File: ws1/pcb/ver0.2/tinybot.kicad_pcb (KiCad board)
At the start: 2 copper layers, 46.7 x 46.2 mm, 19 parts, among them IC1 ATTINY84-P, P1 PWR, P2 Pins Breakout, P3 ICSP, P4 M1, P5 M2, U1 LD1117S33TR, U2 L293D

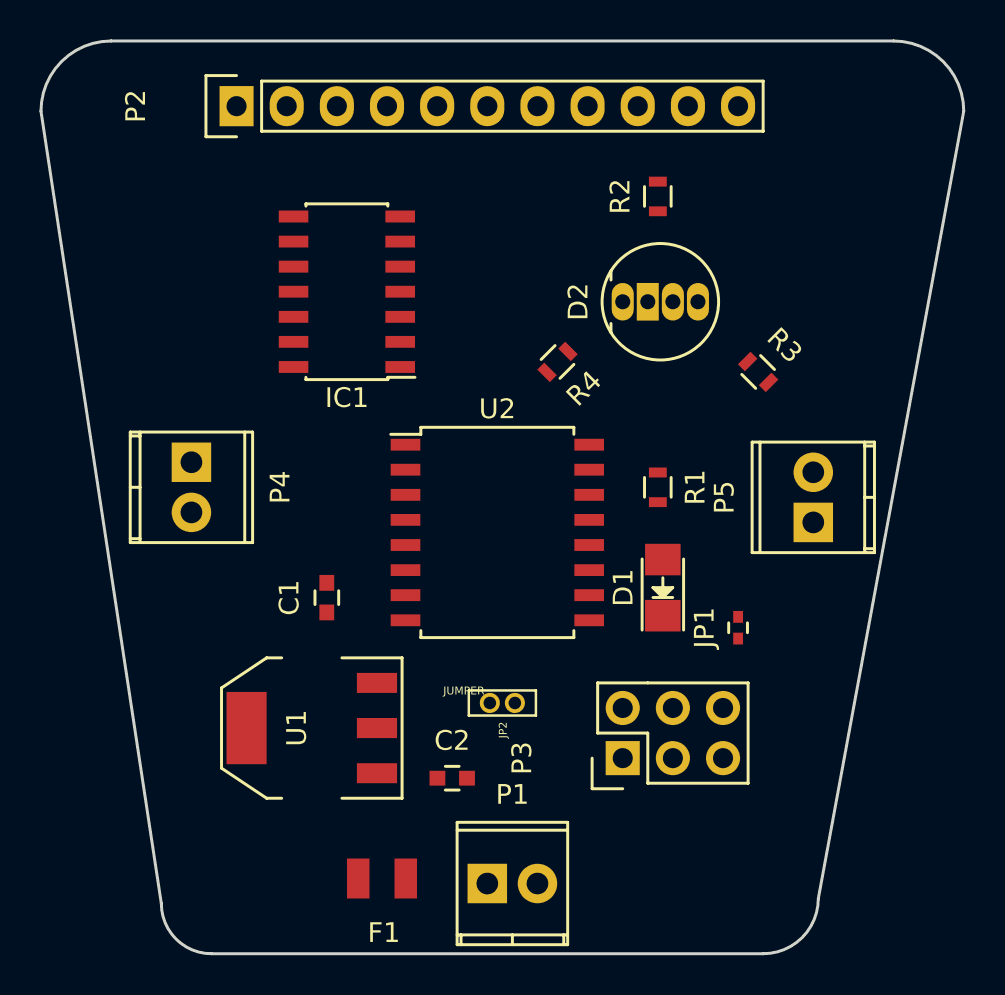
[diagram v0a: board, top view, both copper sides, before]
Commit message: refining PCB
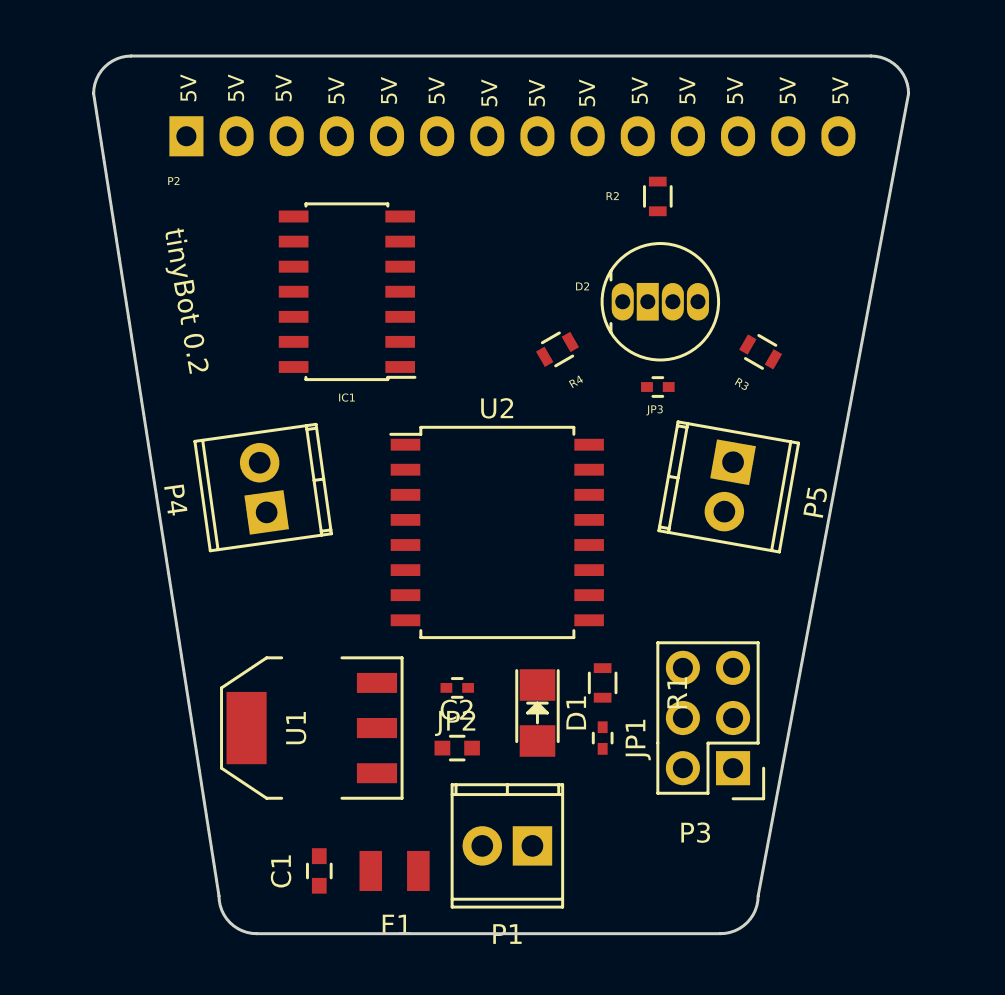
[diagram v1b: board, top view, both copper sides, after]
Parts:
- added JP3: JUMPER, Capacitors_SMD:C_0402, F.Cu at (151.1, 81.5)
- JP2: footprint tinybot:2P-1.27 -> Capacitors_SMD:C_0402
- P2: value Pins Breakout -> Pin Breakout; footprint Pin_Headers:Pin_Header_Straight_1x11 -> tinybot:Pin_Header_Straight_1x14
- moved C1 13.8 mm to (134.0, 106.0)
- moved R1 10.3 mm to (148.3, 96.5)
- moved D1 8.98 mm to (145.0, 98.0), turned to 270 degrees
- moved JP1 8.85 mm to (148.3, 99.3), turned to 270 degrees
- moved P3 5.61 mm to (154.9, 100.8), turned to 180 degrees
- moved P5 5.08 mm to (154.9, 85.3), turned to 260 degrees
- moved P4 4.58 mm to (131.3, 87.9), turned to 98 degrees
- moved P1 2.98 mm to (144.8, 104.8), turned to 180 degrees
- moved P2 2.96 mm to (127.3, 68.8)
- moved JP2 2.41 mm to (141.0, 96.8), turned to 180 degrees
- moved C2 1.55 mm to (141.0, 99.8)
- moved R3 1.02 mm to (156.3, 79.8), turned to 150 degrees
- moved F1 0.74 mm to (137.8, 106.0)
- moved R4 0.63 mm to (146.1, 79.6), turned to 210 degrees
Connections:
- D2 pad 2: GND -> Net-(D2-Pad2)
- P2 pad 10: Net-(IC1-Pad5) -> Net-(IC1-Pad6)
- P2 pad 11: RESET -> DIR2A
- P2 pad 3: DIR1A -> Net-(IC1-Pad13)
- P2 pad 4: DIR1B -> Net-(IC1-Pad12)
- P2 pad 5: MISO -> Net-(IC1-Pad11)
- P2 pad 6: MOSI -> DIR1A
- P2 pad 7: Net-(IC1-Pad6) -> DIR1B
- P2 pad 8: DIR2A -> MISO
- P2 pad 9: DIR2B -> MOSI
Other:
- board size 46.7 x 46.2 mm -> 41.3 x 44.5 mm
- board text added: "5V"
- board text added: "tinyBot 0.2"
